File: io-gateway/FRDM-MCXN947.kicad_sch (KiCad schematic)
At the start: 1 part

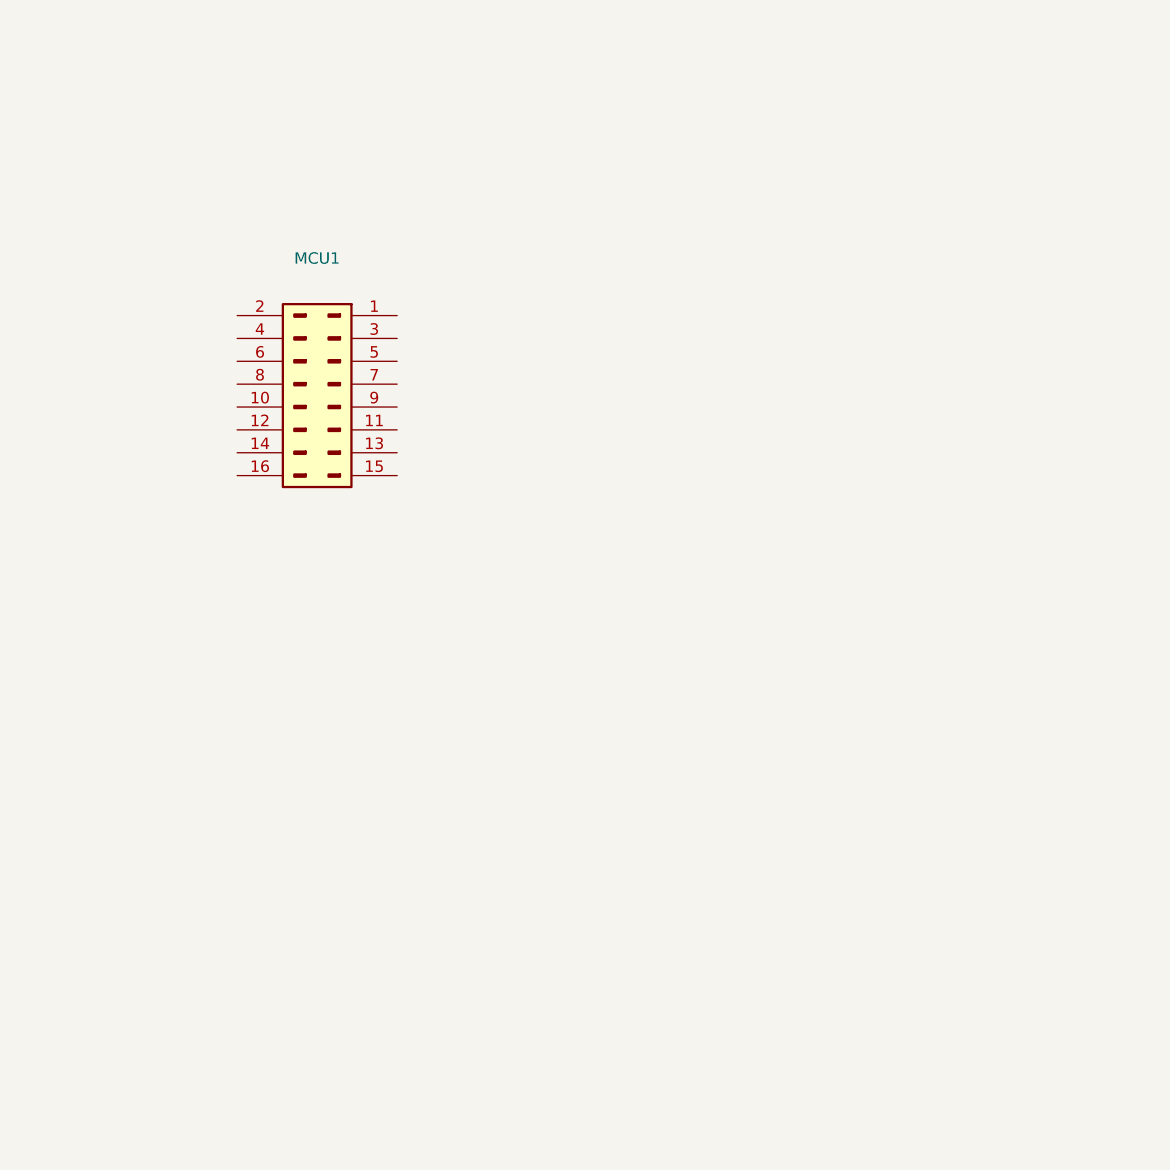
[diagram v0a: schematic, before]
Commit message: update mcu lib
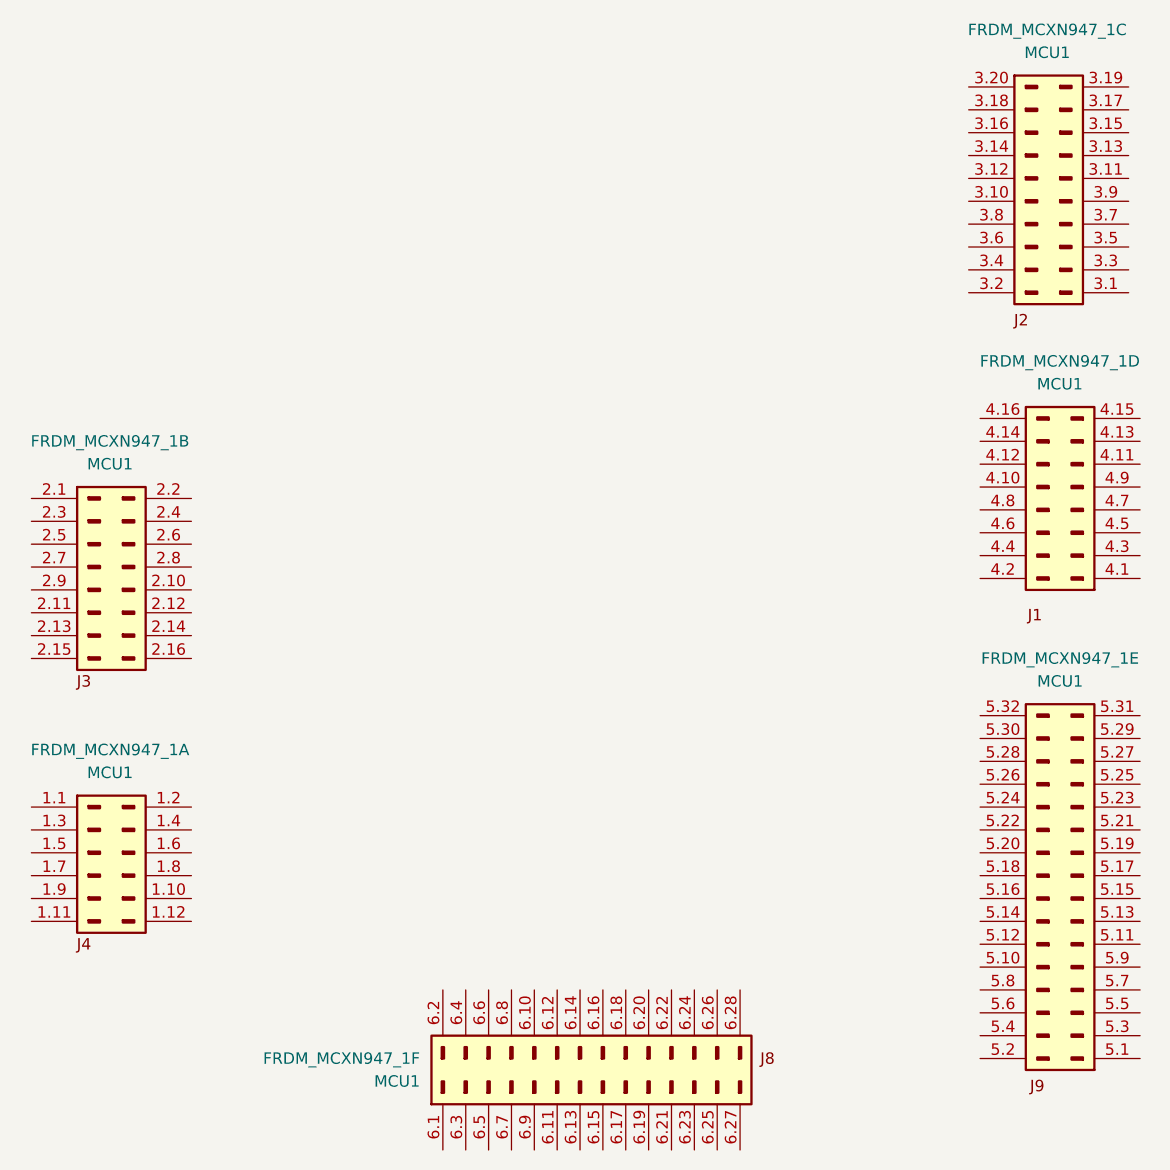
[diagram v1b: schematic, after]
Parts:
- removed MCU1: ~, FRDM-MCXN947:FRDM-MCXN947, symbol FRDM-MCXN947__Shield_Template-altium-import:root_0_mirrored_SSQ-108-03-T-D
- added FRDM_MCXN947_1: MCU1, FRDM-MCXN947:FRDM-MCXN947, symbol FRDM-MCXN947__Shield_Template-altium-import:MCU**
